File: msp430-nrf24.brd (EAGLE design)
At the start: 160 x 100 mm, 12 parts, among them IC1 MSP430G2X53-20N20, IC2 78L33, J1 PWR

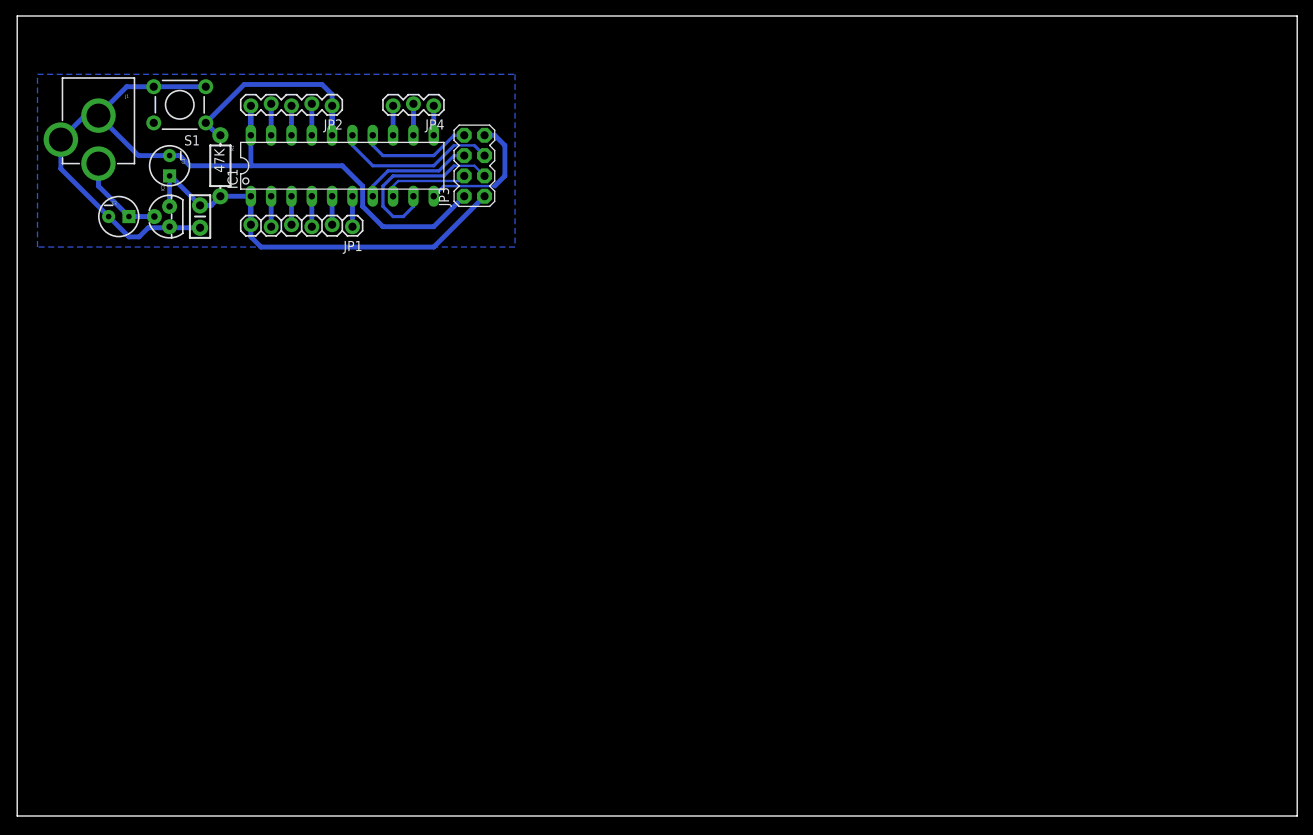
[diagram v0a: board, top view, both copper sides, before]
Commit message: :new: Change board layout
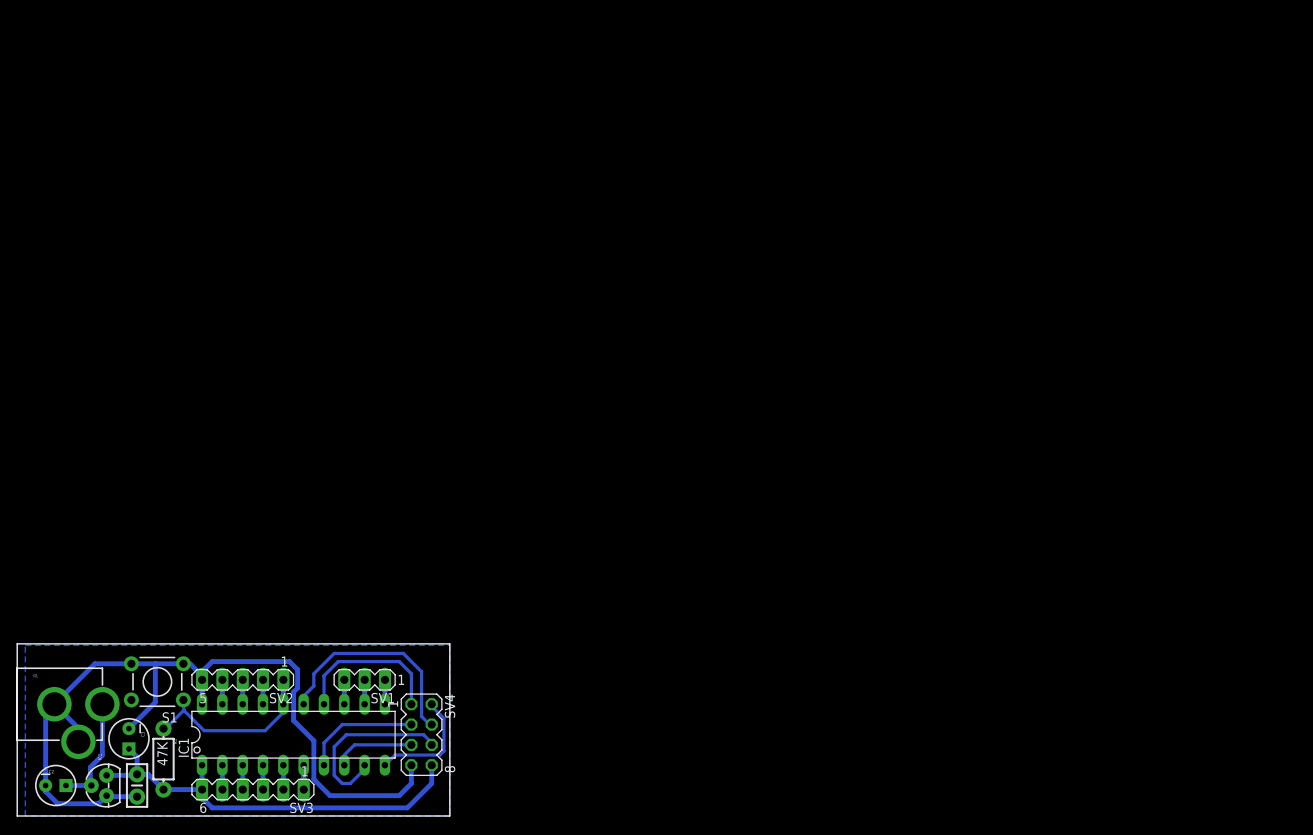
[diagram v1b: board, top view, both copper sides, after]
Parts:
- removed JP1: H1, SparkFun-Connectors:1X06_LOCK
- removed JP2: H2, SparkFun-Connectors:1X05_LOCK
- removed JP3: nRF24L01, SparkFun-Connectors:2X4
- removed JP4: H3, SparkFun-Connectors:1X03_LOCK
- added SV1: (no value), con-lstb:MA03-1
- added SV2: (no value), con-lstb:MA05-1
- added SV3: (no value), con-lstb:MA06-1
- added SV4: (no value), con-lstb:MA04-2
- moved J1 82.3 mm to (-3.05, 14.0), turned to 270 degrees
- moved R1 74.5 mm to (18.3, 7.11)
- moved S1 72.2 mm to (17.5, 16.8)
- moved C3 71.8 mm to (14.0, 9.65)
- moved C1 71.6 mm to (15.0, 3.81)
- moved C2 71.6 mm to (4.83, 3.81)
- moved IC2 71.6 mm to (11.2, 3.81)
- moved IC1 71.4 mm to (34.5, 10.2)
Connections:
- net CE: now also SV4.5; no longer JP3.4
- net CSN: now also SV4.6; no longer JP3.3
- net GND: now also SV2.5, SV4.7; no longer JP2.5, JP3.2
- net IRQ: now also SV4.2; no longer JP3.7
- net MISO: now also SV4.1; no longer JP3.8
- net MOSI: now also SV4.4; no longer JP3.5
- net P1.0: now also SV3.5; no longer JP1.5
- net P1.1: now also SV3.4; no longer JP1.4
- net P1.2: now also SV3.3; no longer JP1.3
- net P1.3: now also SV3.2; no longer JP1.2
- net P1.4: now also SV3.1; no longer JP1.1
- net P2.3: now also SV1.1; no longer JP4.1
- net P2.4: now also SV1.2; no longer JP4.2
- net P2.5: now also SV1.3; no longer JP4.3
- net P2.6: now also SV2.4; no longer JP2.4
- net P2.7: now also SV2.3; no longer JP2.3
- net RST: now also SV2.1; no longer JP2.1
- net SCK: now also SV4.3; no longer JP3.6
- net TEST: now also SV2.2; no longer JP2.2
- net VCC: now also SV3.6, SV4.8; no longer JP1.6, JP3.1
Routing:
- net MOSI: track 20.4 -> 27.1 mm
- net RST: track 29.5 -> 23.3 mm
- net MISO: track 14.3 -> 19.7 mm
- net VCC: track 57.6 -> 53.4 mm
- net GND: track 111.9 -> 108.2 mm
- net N$1: track 11.4 -> 14.0 mm
- net IRQ: track 16.8 -> 14.6 mm
- net CSN: track 24.2 -> 22.5 mm
- net P1.1: track 4.07 -> 3.05 mm
- net P2.4: track 3.94 -> 3.05 mm
- net P2.6: track 3.94 -> 3.05 mm
- net TEST: track 3.94 -> 3.05 mm
- net P1.0: track 3.82 -> 3.05 mm
- net P1.4: track 3.81 -> 3.05 mm
- net P1.2: track 3.81 -> 3.05 mm
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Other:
- board size 160 x 100 mm -> 54.1 x 21.5 mm
